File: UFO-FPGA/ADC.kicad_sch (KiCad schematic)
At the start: 1 part, among them U12 MAX11116AUT+T

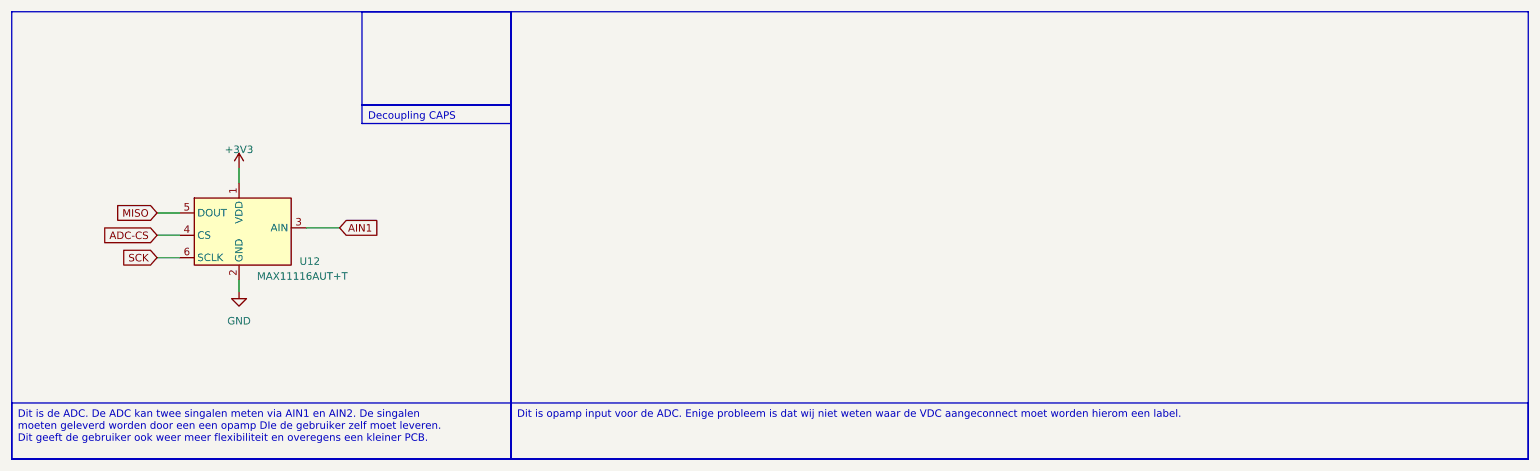
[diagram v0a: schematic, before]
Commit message: PCB
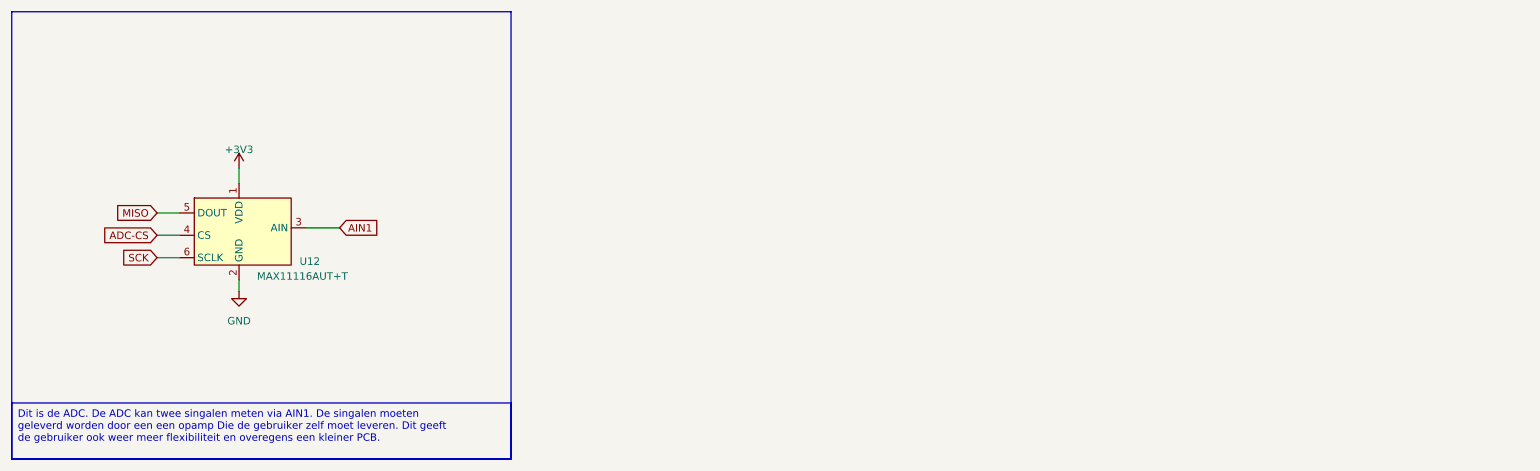
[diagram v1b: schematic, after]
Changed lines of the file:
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@@
     (stroke (width 0) (type default))
-  )
-  (rectangle (start 78.74 18.415) (end 104.14 34.29)
-    (stroke (width 0) (type default))
-    (fill (type none))
   )
   (rectangle (start 19.05 18.415) (end 104.14 94.615)
@@
     (fill (type none))
   )
-  (rectangle (start 104.14 18.415) (end 277.495 94.615)
-    (stroke (width 0) (type default))
-    (fill (type none))
-  )
-  (text_box "Dit is opamp input voor de ADC. Enige probleem is dat wij niet weten waar de VDC aangeconnect moet worden hierom een label.\n"
-    (at 104.14 85.09 0) (size 173.355 9.525)
-    (stroke (width 0) (type default))
-    (fill (type none))
-    (effects (font (size 1.27 1.27)) (justify left top))
-  )
-  (text_box "Decoupling CAPS"
-    (at 78.74 34.29 0) (size 25.4 3.175)
-    (stroke (width 0) (type default))
-    (fill (type none))
-    (effects (font (size 1.27 1.27)) (justify left top))
-  )
-  (text_box "Dit is de ADC. De ADC kan twee singalen meten via AIN1 en AIN2. De singalen moeten geleverd worden door een een opamp DIe de gebruiker zelf moet leveren. Dit geeft de gebruiker ook weer meer flexibiliteit en overegens een kleiner PCB."
+  (text_box "Dit is de ADC. De ADC kan twee singalen meten via AIN1. De singalen moeten geleverd worden door een een opamp Die de gebruiker zelf moet leveren. Dit geeft de gebruiker ook weer meer flexibiliteit en overegens een kleiner PCB."
     (at 19.05 85.09 0) (size 85.09 9.525)
     (stroke (width 0) (type default))
